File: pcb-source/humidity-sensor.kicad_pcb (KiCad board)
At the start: 2 copper layers, 38.7 x 24.2 mm, 40 parts, among them J1 Conn_ARM_JTAG_SWD_10, Q1 Q_NMOS_GSD, Q2 Q_NMOS_GSD, U1 STM32L051C8Tx, U2 SHTC3, U3 SYN115, Y1 13.56MHz, Y2 DNU

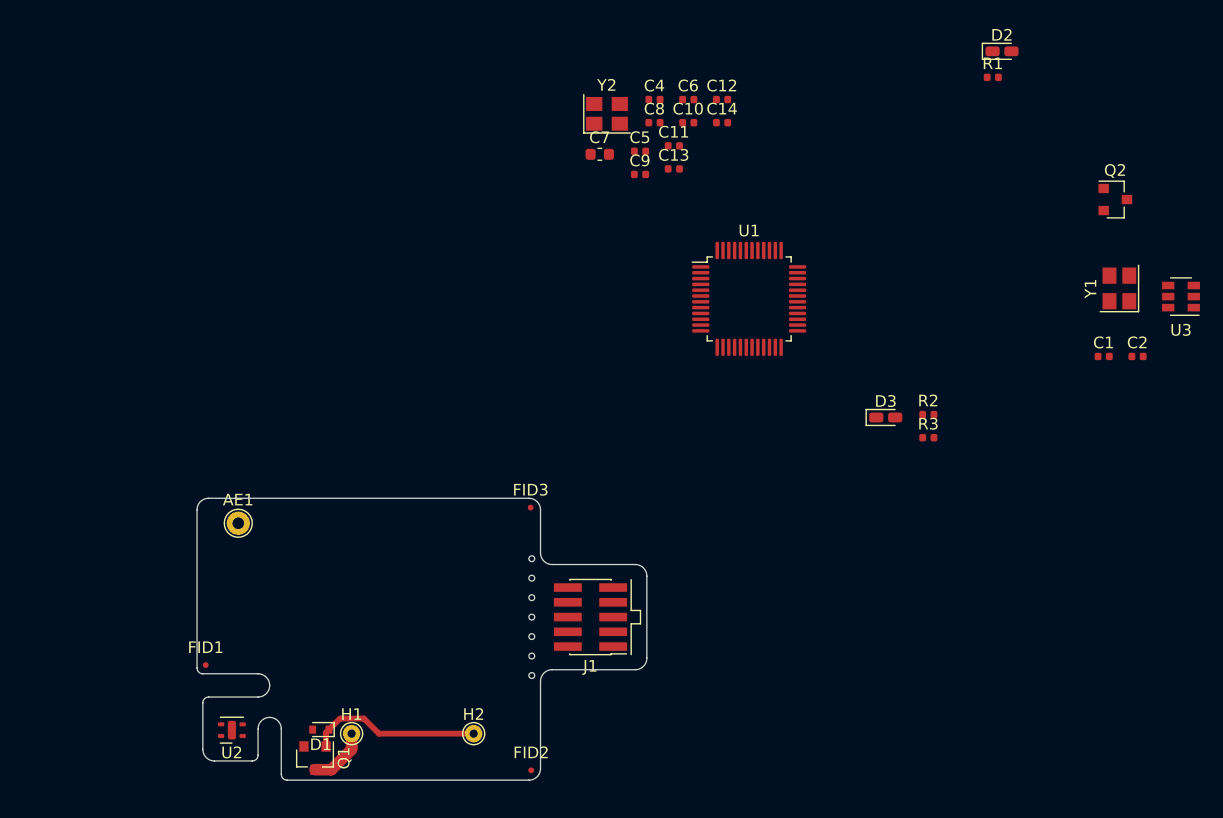
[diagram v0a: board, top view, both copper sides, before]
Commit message: Work on schem and PCB
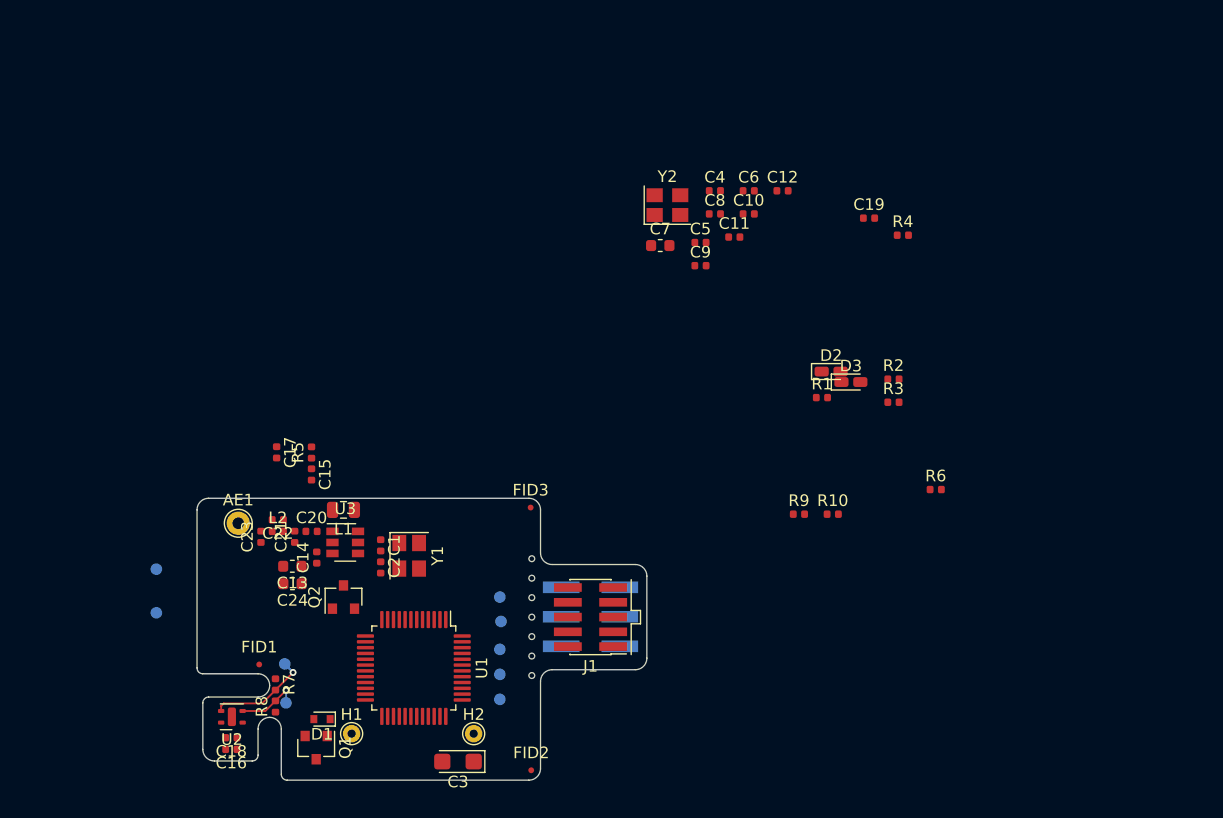
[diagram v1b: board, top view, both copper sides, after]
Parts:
- added C13: 10uF, Capacitor_SMD:C_0603_1608Metric, F.Cu at (86.8, 73.0)
- added C14: 0.1uF, Capacitor_SMD:C_0402_1005Metric, F.Cu at (89.0, 72.3)
- added C15: 100pF C0G, Capacitor_SMD:C_0402_1005Metric, F.Cu at (88.5, 65.2)
- added C17: DNU, Capacitor_SMD:C_0402_1005Metric, F.Cu at (85.5, 63.2)
- added C19: DNU, Capacitor_SMD:C_0402_1005Metric, F.Cu at (136.5, 43.1)
- added C20: 12pF C0G, Capacitor_SMD:C_0402_1005Metric, F.Cu at (88.5, 70.0)
- added C21: DNU, Capacitor_SMD:C_0402_1005Metric, F.Cu at (87.0, 70.5)
- added C22: DNU, Capacitor_SMD:C_0402_1005Metric, F.Cu at (85.6, 69.0)
- added C23: 4.7pF C0G, Capacitor_SMD:C_0402_1005Metric, F.Cu at (84.2, 70.5)
- added C24: 10uF, Capacitor_SMD:C_0603_1608Metric, F.Cu at (86.9, 74.5)
- added C3: 22uF 10V, Capacitor_Tantalum_SMD:CP_EIA-3216-18_Kemet-A, F.Cu at (101.1, 89.8)
- added J2: Conn_02x03_Odd_Even, Connector_PinHeader_2.54mm:PinHeader_2x03_P2.54mm_Vertical_SMD, B.Cu at (112.5, 77.4)
- added L1: 820nH, Inductor_SMD:L_0805_2012Metric, F.Cu at (91.2, 68.2)
- added L2: 68nH, Inductor_SMD:L_0402_1005Metric, F.Cu at (85.6, 70.0)
- added R10: 0R, Resistor_SMD:R_0402_1005Metric, F.Cu at (133.3, 68.6)
- added R4: 100K, Resistor_SMD:R_0402_1005Metric, F.Cu at (139.4, 44.6)
- added R5: 0R, Resistor_SMD:R_0402_1005Metric, F.Cu at (88.5, 63.3)
- added R6: 100K, Resistor_SMD:R_0402_1005Metric, F.Cu at (142.2, 66.5)
- added R7: 10K, Resistor_SMD:R_0402_1005Metric, F.Cu at (85.4, 83.2)
- added R8: 10K, Resistor_SMD:R_0402_1005Metric, F.Cu at (85.4, 85.1)
- added R9: 0R, Resistor_SMD:R_0402_1005Metric, F.Cu at (130.4, 68.6)
- added TP1: TP_RF_EN, TestPoint:TestPoint_Pad_D1.0mm, B.Cu at (75.2, 73.3)
- added TP2: TP_RF_DATA, TestPoint:TestPoint_Pad_D1.0mm, B.Cu at (75.2, 77.0)
- added TP3: TP_HUM_SDA, TestPoint:TestPoint_Pad_D1.0mm, B.Cu at (86.2, 81.5)
- added TP4: TP_HUM_SCL, TestPoint:TestPoint_Pad_D1.0mm, B.Cu at (86.3, 84.8)
- added TP5: TP_UART_RX, TestPoint:TestPoint_Pad_D1.0mm, B.Cu at (104.8, 77.8)
- added TP6: TP_UART_TX, TestPoint:TestPoint_Pad_D1.0mm, B.Cu at (104.7, 82.3)
- added TP7: TP_DEBUG_1, TestPoint:TestPoint_Pad_D1.0mm, B.Cu at (104.7, 75.7)
- added TP8: TP_DEBUG_2, TestPoint:TestPoint_Pad_D1.0mm, B.Cu at (104.7, 84.5)
- added TP9: TP_DEBUG_3, TestPoint:TestPoint_Pad_D1.0mm, B.Cu at (104.7, 80.2)
- moved U3 74.9 mm to (91.4, 71.0), turned to 0 degrees
- moved Q2 74.7 mm to (91.2, 75.7), turned to 90 degrees
- moved C18 67.7 mm to (81.6, 87.8), turned to 180 degrees
- moved C2 67.6 mm to (94.5, 73.2), turned to 270 degrees
- moved Y1 65.3 mm to (96.9, 72.2), turned to 270 degrees
- moved C1 64.3 mm to (94.5, 71.2), turned to 270 degrees
- moved C16 62.8 mm to (81.6, 88.8), turned to 180 degrees
- moved U1 42.9 mm to (97.3, 81.8), turned to 270 degrees
- moved D2 31.2 mm to (133.2, 56.3)
- moved R1 31.2 mm to (132.4, 58.5)
- moved C12 9.42 mm to (129.0, 40.8)
- moved C10 9.42 mm to (126.1, 42.7)
- moved C4 9.42 mm to (123.2, 40.8)
- moved C6 9.42 mm to (126.1, 40.8)
- moved C7 9.42 mm to (118.5, 45.5)
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- renumbered C13 to C16, C14 to C18
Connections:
- C16 pad 1: Net-(C13-Pad1) -> Net-(C16-Pad1)
- C16 pad 2: Net-(C13-Pad2) -> GND
- C18 pad 1: Net-(C14-Pad1) -> Net-(C16-Pad1)
- C18 pad 2: Net-(C14-Pad2) -> GND
- U1 pad 10: Net-(U1-Pad10) -> Net-(R3-Pad1)
- U1 pad 11: Net-(U1-Pad11) -> Net-(R1-Pad1)
- U1 pad 16: Net-(U1-Pad16) -> /RF_EN
- U1 pad 17: Net-(U1-Pad17) -> /RF_DATA
- U1 pad 21: Net-(U1-Pad21) -> /UART_TX
- U1 pad 22: Net-(U1-Pad22) -> /UART_RX
- U1 pad 26: Net-(U1-Pad26) -> /HUM_SCL
- U1 pad 27: Net-(U1-Pad27) -> /HUM_SDA
- U1 pad 43: Net-(U1-Pad43) -> /DEBUG_1
- U1 pad 45: Net-(U1-Pad45) -> /DEBUG_2
- U1 pad 46: Net-(U1-Pad46) -> /DEBUG_3
- U2 pad 1: VCC -> Net-(C16-Pad1)
- U2 pad 2: Net-(U2-Pad2) -> /HUM_SCL
- U2 pad 3: Net-(U2-Pad3) -> /HUM_SDA
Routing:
- net VCC: track 14.9 -> 0.00 mm
- net /HUM_SDA: track 0.00 -> 9.46 mm, vias 0 -> 1
- net /HUM_SCL: track 0.00 -> 5.57 mm, vias 0 -> 1
- net Net-(H1-Pad1): track 5.22 -> 0.00 mm
- net /UART_RX: track 0.00 -> 0.67 mm
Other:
- net class Default: clearance 0.2 -> 0.1524; trace_width 0.25 -> 0.2; via_dia 0.8 -> 0.6; via_drill 0.4 -> 0.3
- rule pad_to_mask_clearance: 0.051 -> 0
- rule solder_mask_min_width: 0.25 -> 0.2
- rule trace_clearance: 0.2 -> 0.1524
- rule trace_min: 0.2 -> 0.1524
- rule via_min_size: 0.4 -> 0.6

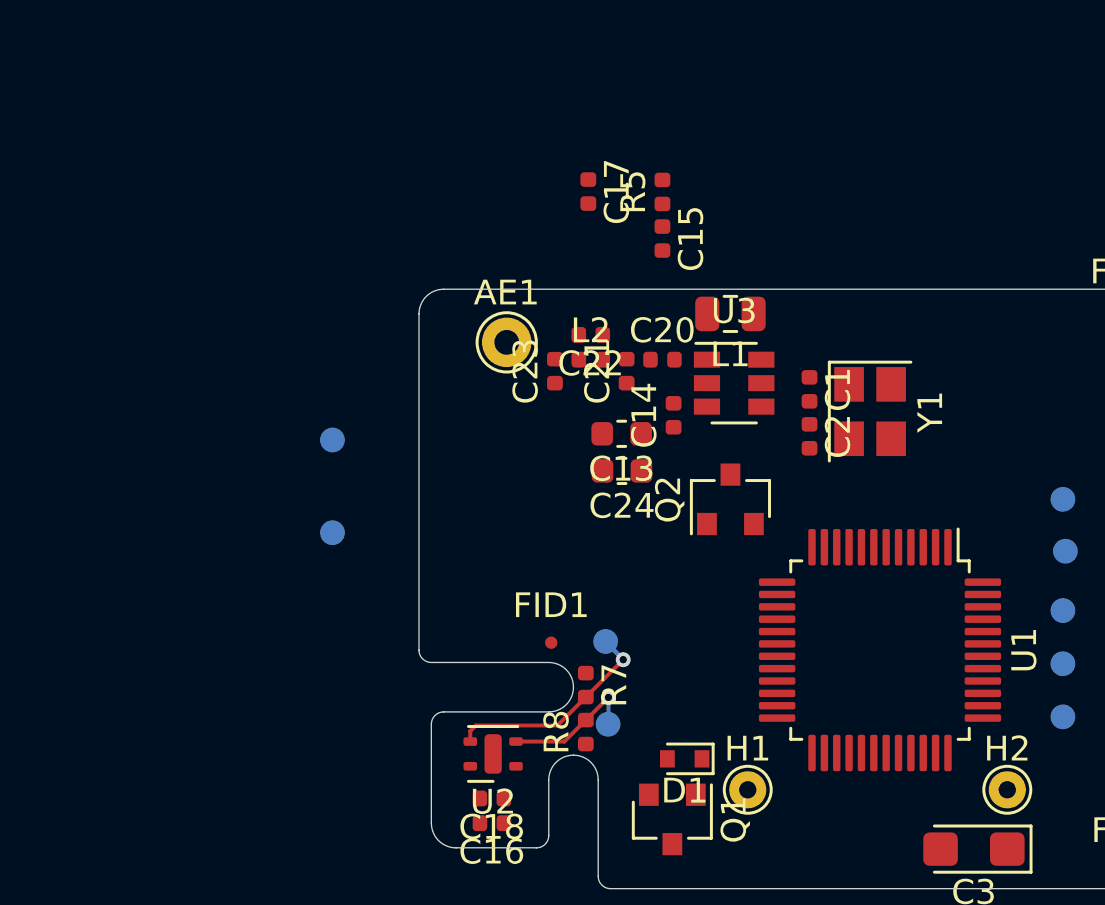
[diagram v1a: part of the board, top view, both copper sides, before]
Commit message: Work on layout
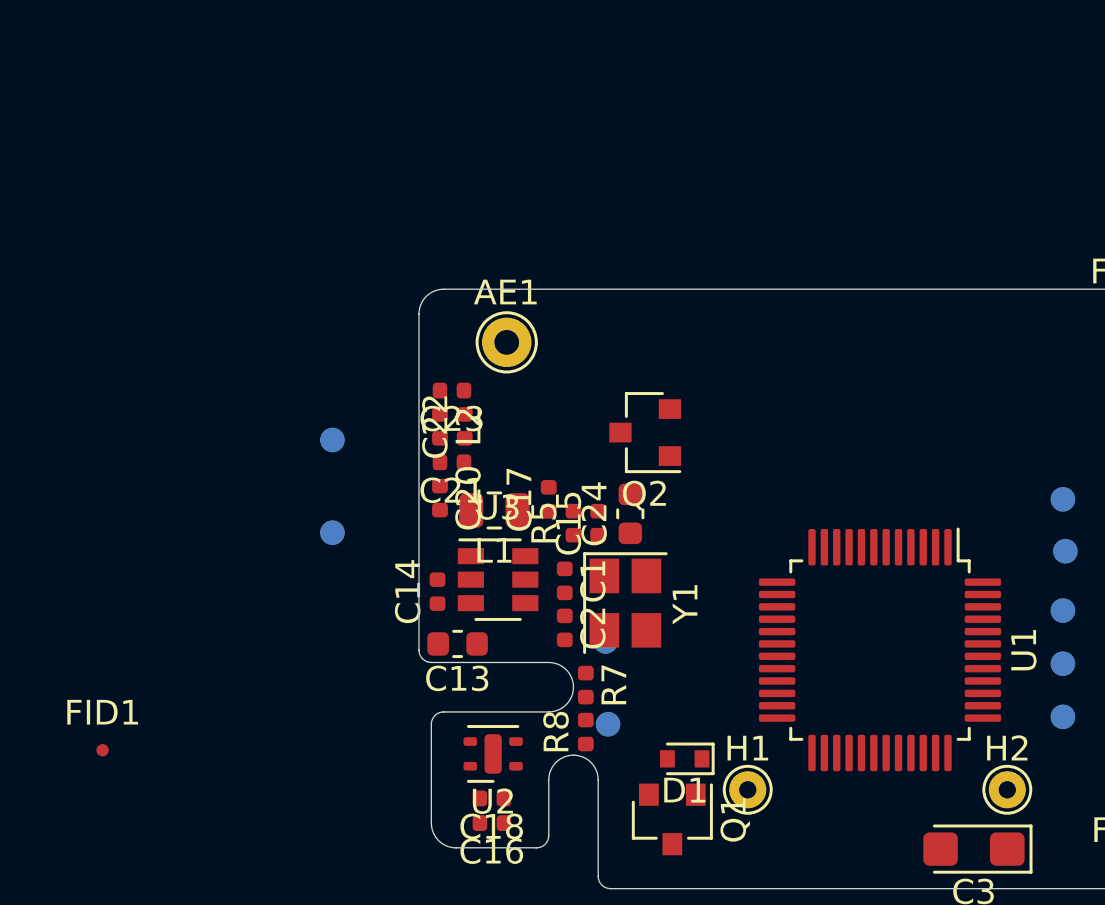
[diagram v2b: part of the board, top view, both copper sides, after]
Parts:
- moved FID1 18.7 mm to (65.8, 85.8)
- moved R5 13.9 mm to (84.9, 76.7)
- moved C1 12.6 mm to (84.5, 79.0)
- moved C2 12.6 mm to (84.5, 80.9)
- moved Y1 12.6 mm to (87.0, 79.9)
- moved C17 12.6 mm to (83.9, 75.7), turned to 90 degrees
- moved U3 12.4 mm to (81.8, 79.0)
- moved L1 12.4 mm to (81.7, 76.2)
- moved C14 11.9 mm to (79.4, 79.4)
- moved C15 11.8 mm to (85.9, 76.7), turned to 90 degrees
- moved C13 10.8 mm to (80.2, 81.5)
- moved C20 10.6 mm to (79.5, 75.7), turned to 270 degrees
- moved C21 7.97 mm to (80.0, 74.2), turned to 180 degrees
- moved L2 6.67 mm to (79.5, 72.8), turned to 270 degrees
- moved C22 6.30 mm to (80.5, 72.8), turned to 90 degrees
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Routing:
- net /HUM_SDA: track 9.46 -> 0.00 mm, vias 1 -> 0
- net /HUM_SCL: track 5.57 -> 0.00 mm, vias 1 -> 0
